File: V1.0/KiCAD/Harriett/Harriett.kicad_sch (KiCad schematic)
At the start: 21 parts, among them J1 Conn_02x08_Odd_Even, Q1 TP0604, Q2 2N3904, U1 ButtonPad_2x2, U2 DFRobotMP3PlayerMini, U4 BlackPill_F401CC

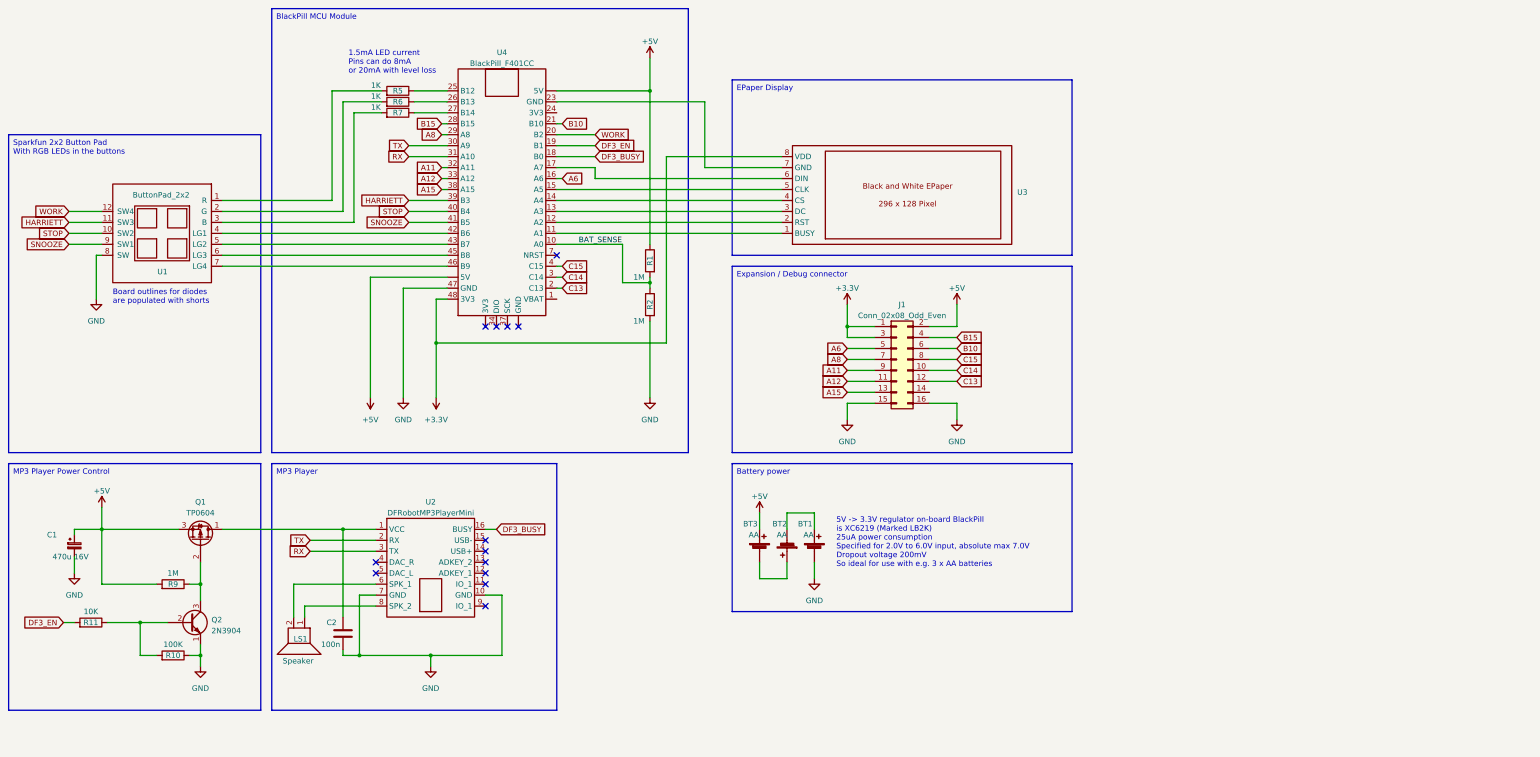
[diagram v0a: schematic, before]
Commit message: Catchup
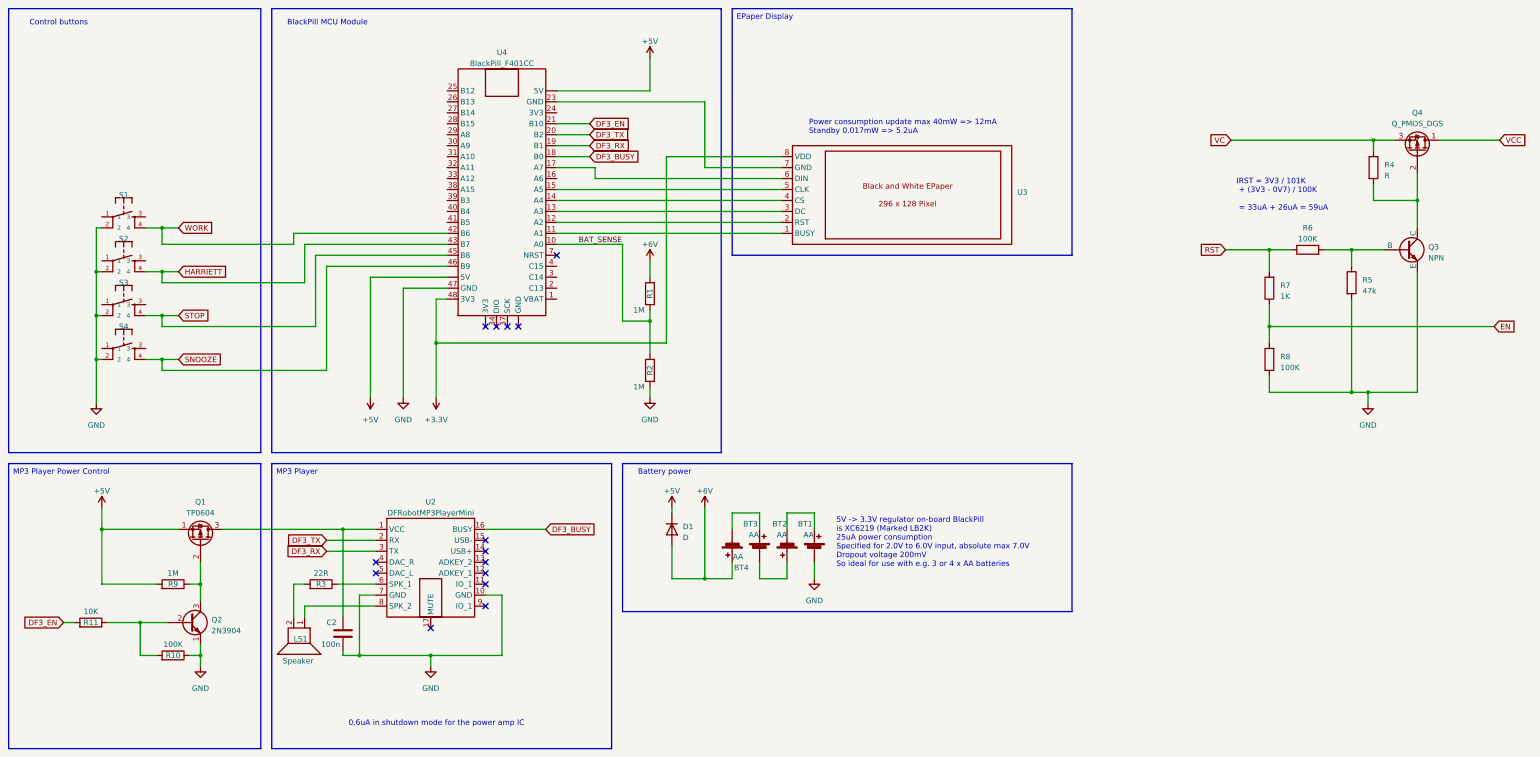
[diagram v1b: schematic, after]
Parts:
- removed C1: 470u 16V, symbol Device:C_Polarized_Small
- removed J1: Conn_02x08_Odd_Even, symbol Connector_Generic:Conn_02x08_Odd_Even
- removed U1: ButtonPad_2x2, symbol UKMaker:ButtonPad_2x2
- added BT4: AA, symbol Device:Battery_Cell
- added D1: D, symbol Device:D
- added Q3: NPN, symbol Simulation_SPICE:NPN
- added Q4: Q_PMOS_DGS, symbol Device:Q_PMOS_DGS
- added R3: 22R, symbol Device:R
- added R4: R, symbol Device:R
- added R8: 100K, symbol Device:R
- added S1, S2, S3, S4: ~, SparkFun-KSA_SEALED_TAC_SWITCH, symbol Sparkfun:TAC_SWITCHKSA_SEALED
- Q1: symbol Device:Q_PMOS_DGS -> Device:Q_PMOS_SGD
- R5: value 1K -> 47k
- R6: value 1K -> 100K
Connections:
- net B10 is gone; now on net DF3_EN: U4.21 (B10)
- net +5V: now also Q1.1 (S), D1.1 (K); no longer BT3.1 (+), Q1.3 (S), R1.1
- net DF3_EN: no longer U4.19 (B1)
- net GND: now also R5.2, Q3.3 (E), R8.1, S1.2, S2.2, S3.2, S4.2
- net HARRIETT: now also U4.43 (B7), S2.4; no longer U4.39 (B3)
- net SNOOZE: now also U4.46 (B9), S4.4; no longer U4.41 (B5)
- net STOP: now also U4.45 (B8), S3.4; no longer U4.40 (B4)
- net WORK: now also U4.42 (B6), S1.4; no longer U4.20 (B2)
- net at C2.1, U2.1 (VCC): now also Q1.3 (D); no longer Q1.1 (D)
- net at U2.6 (SPK_1): now also R3.1; no longer LS1.2
- net at R5.1: now also R6.2, Q3.2 (B); no longer U4.25 (B12)
- net at U4.26 (B13): no longer R6.1
- net at U4.27 (B14): no longer R7.1
- net RST: now reaches R7.2
- net RST: now also R6.1
- net A11: no longer names the net of U4.32 (A11)
- net A12: no longer names the net of U4.33 (A12)
- net A15: no longer names the net of U4.38 (A15)
- net A6: no longer names the net of U4.16 (A6)
- net A8: no longer names the net of U4.29 (A8)
- net B15: no longer names the net of U4.28 (B15)
- net C13: no longer names the net of U4.2 (C13)
- net C14: no longer names the net of U4.3 (C14)
- net C15: no longer names the net of U4.4 (C15)
- net RX: no longer names the net of U4.31 (A10)
- net RX: no longer U2.3 (TX)
- net TX: no longer names the net of U4.30 (A9)
- net TX: no longer U2.2 (RX)
- new net: BT3.1 (+), BT4.2 (-)
- new net: Q3.1 (C), Q4.2 (G), R4.2
- new net: LS1.2, R3.2
- new net +6V: BT4.1 (+), D1.2 (A), R1.1
- new net DF3_RX: U2.3 (TX), U4.19 (B1)
- new net DF3_TX: U2.2 (RX), U4.20 (B2)
- new net EN: R7.1, R8.2
- new net VC: Q4.3 (S), R4.1
- new net VCC: Q4.1 (D)
- no-connect marks 13 -> 14
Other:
- note added: "0.6uA in shutdown mode for the power amp IC"
- note added: "5V -> 3.3V regulator on-board BlackPill is XC6219 (Marked LB2K) 25uA power consumption Specified for 2.0V to 6.0V input, absolute max 7.0V Dropout voltage 200mV So ideal for use with e.g. 3 or 4 x AA batteries"
- note added: "IRST = 3V3 / 101K + (3V3 - 0V7) / 100K = 33uA + 26uA = 59uA"
- note added: "Power consumption update max 40mW => 12mA Standby 0.017mW => 5.2uA"
- note removed: "1.5mA LED current Pins can do 8mA or 20mA with level loss"
- note removed: "5V -> 3.3V regulator on-board BlackPill is XC6219 (Marked LB2K) 25uA power consumption Specified for 2.0V to 6.0V input, absolute max 7.0V Dropout voltage 200mV So ideal for use with e.g. 3 x AA batteries"
- note removed: "Board outlines for diodes are populated with shorts"
- moved on the sheet: R1, R2

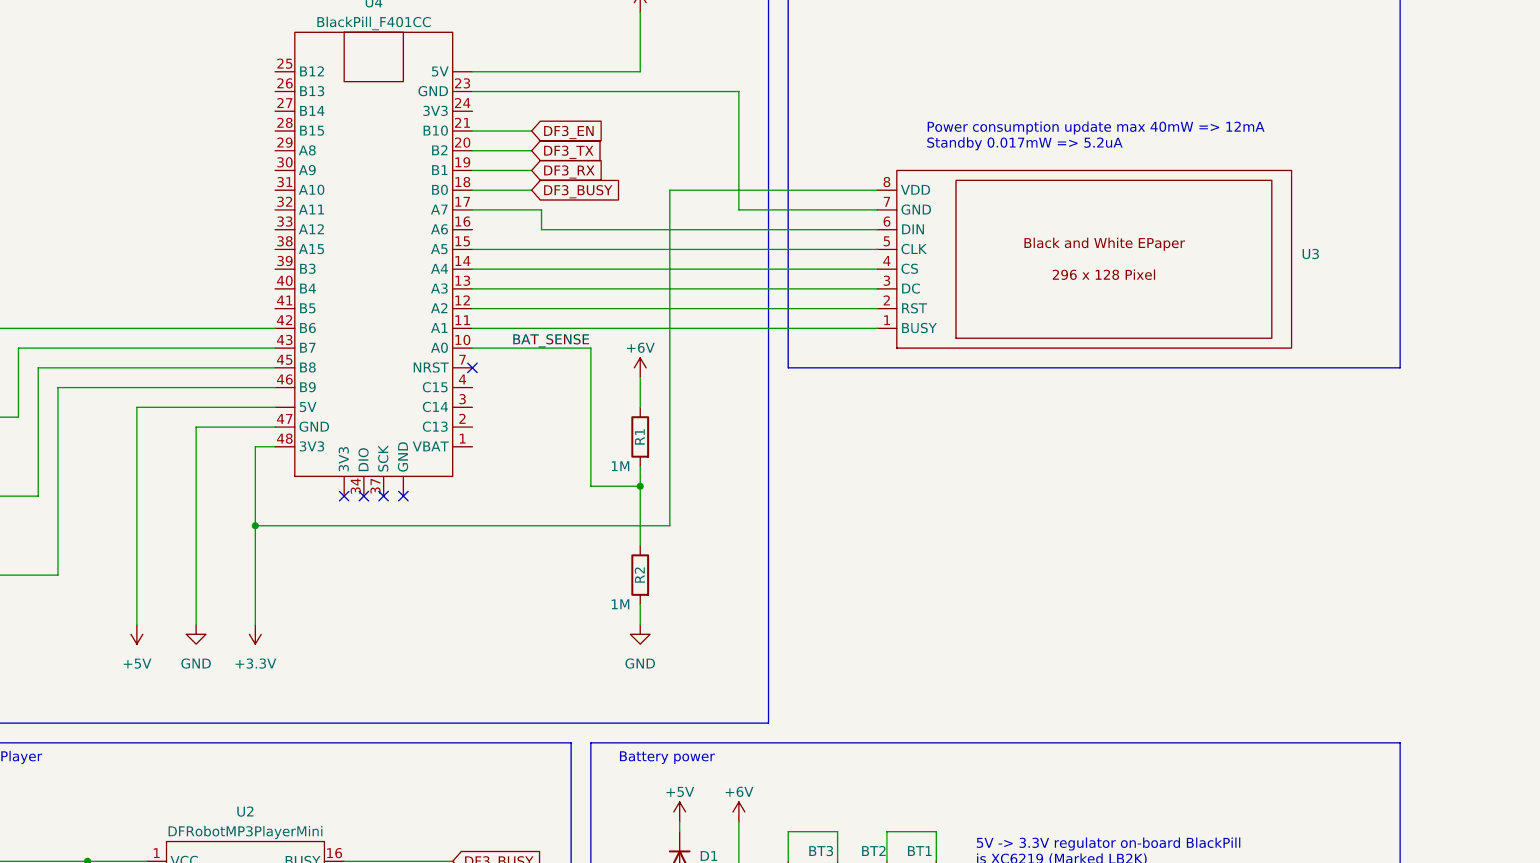
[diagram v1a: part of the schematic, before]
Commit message: Various updates backported from EDAWin - may be broken
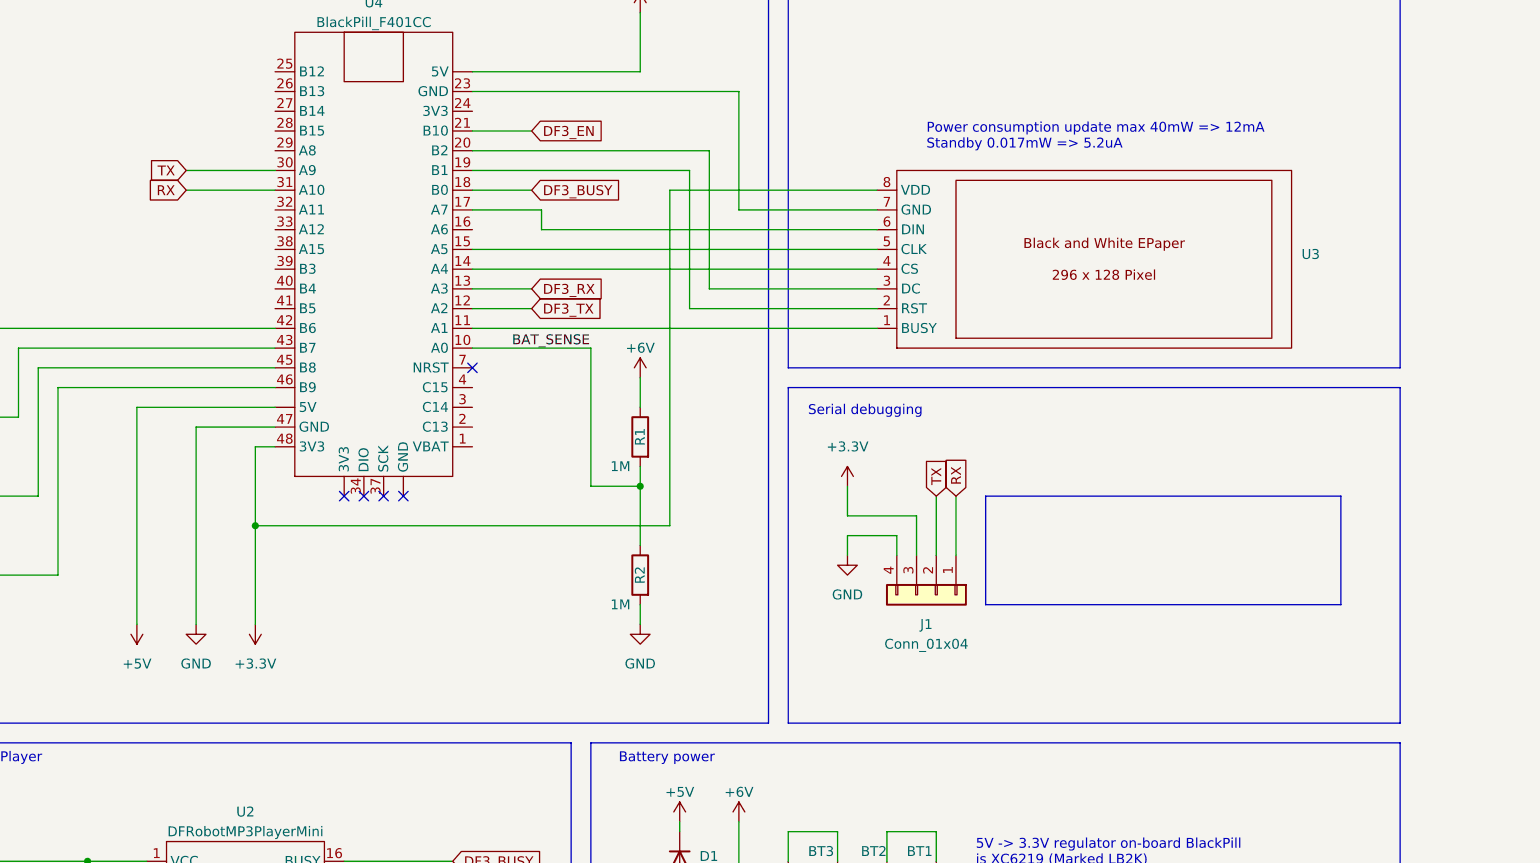
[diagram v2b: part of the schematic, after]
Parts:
- added J1: Conn_01x04, symbol Connector_Generic:Conn_01x04
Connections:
- net +3.3V: now also J1.3 (Pin_3)
- net DF3_RX: now also U4.13 (A3); no longer U4.19 (B1)
- net DF3_TX: now also U4.12 (A2); no longer U4.20 (B2)
- net GND: now also J1.4 (Pin_4)
- net at U3.2 (RST): now also U4.19 (B1); no longer U4.12 (A2)
- net at U3.3 (DC): now also U4.20 (B2); no longer U4.13 (A3)
- net TX: now reaches U4.30 (A9)
- net TX: now also J1.2 (Pin_2)
- net RX: now reaches U4.31 (A10)
- net RX: now also J1.1 (Pin_1)
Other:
- note added: "Serial debugging"
